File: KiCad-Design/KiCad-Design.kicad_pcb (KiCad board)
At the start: 2 copper layers, 35 x 35 mm, 66 parts, among them J1 USB_B_Micro, J2 Battery, J3 Ext, J4 OLED, Q1 SI2301, Q2 SI2301, Q3 SI2307CDS-T1-GE3, Q4 UMH3N, SW1 MCU BLE Adv, SW2 MCU FLASH, SW3 MCU RESET, U1 PMBT3904, U10 HDC1080, U2 BME280, U3 CP2104, U4 LTC4054ES5-4.2, U7 BME680, U8 AP2112K-3.3, U9 ttgo-32-micro-symbols

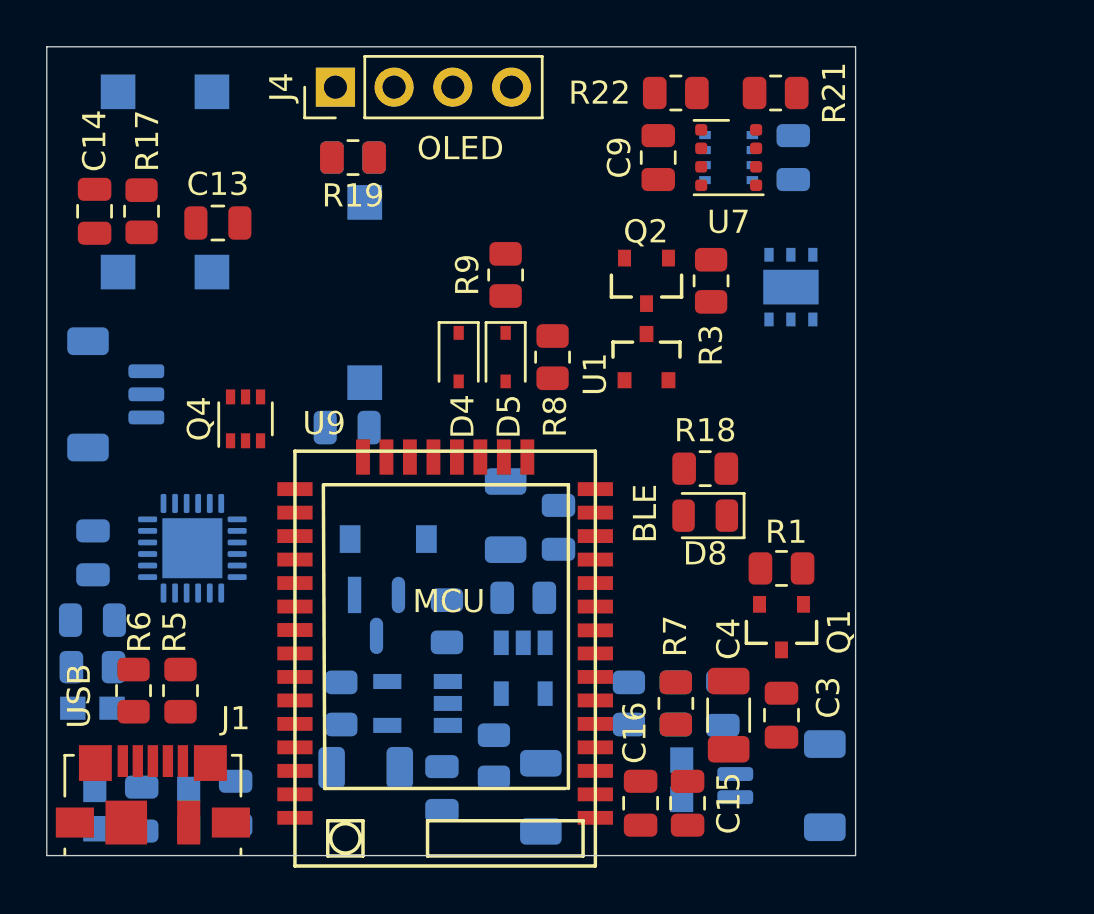
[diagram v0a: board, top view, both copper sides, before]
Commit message: PCB: Updating the PCB design file :)
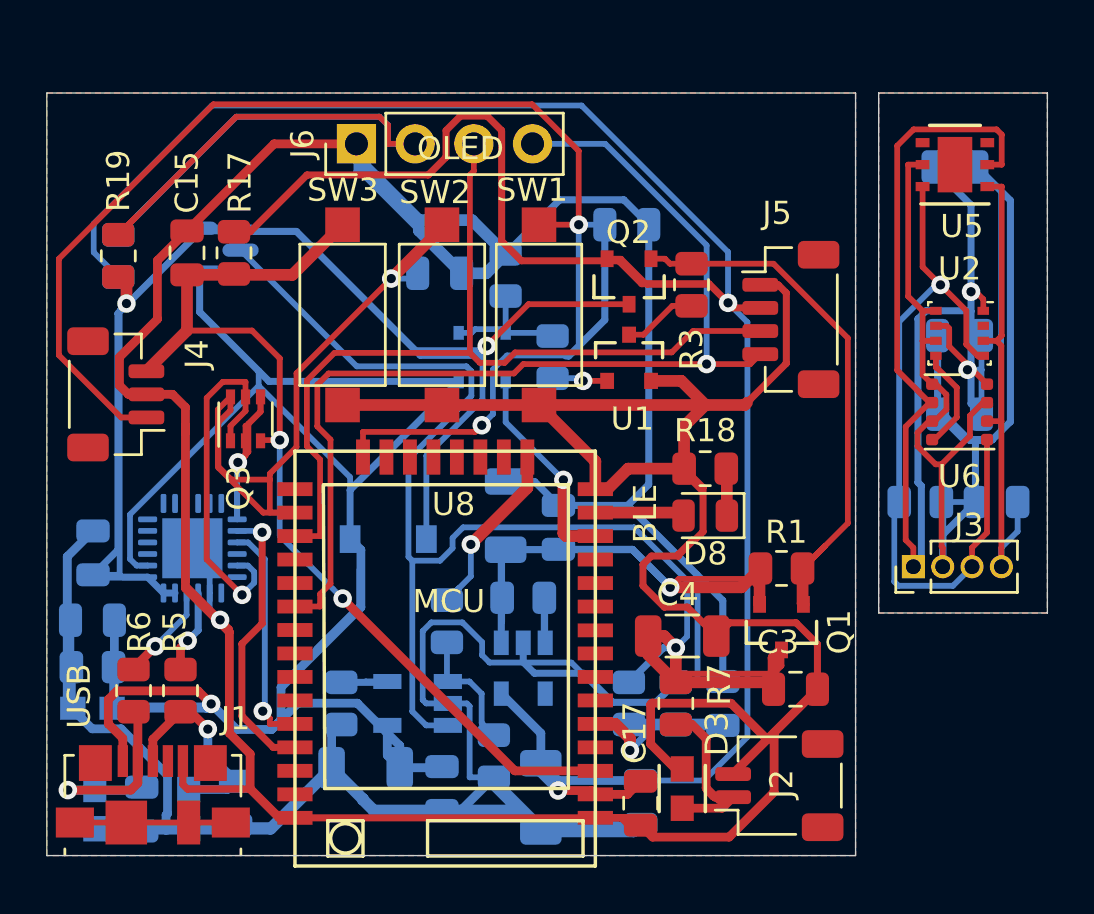
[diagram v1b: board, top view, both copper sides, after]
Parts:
- removed R21, R22: 4.7K, Resistor_SMD:R_0805_2012Metric
- removed U10: HDC1080, Package_SON:Texas_PWSON-N6
- removed the U7 at (254.5, 129.8)
- added C10: 100nF, Capacitor_SMD:C_0805_2012Metric, B.Cu at (264.5, 140.9)
- added J3: SENSOR, Connector_PinHeader_1.27mm:PinHeader_1x04_P1.27mm_Vertical, F.Cu at (262.5, 147.5)
- added J5: SENSORS, Connector_JST:JST_SH_BM04B-SRSS-TB_1x04-1MP_P1.00mm_Vertical, F.Cu at (257.2, 136.8)
- added R14: 4.7K, Resistor_SMD:R_0805_2012Metric, B.Cu at (266.1, 144.7)
- added R15: 4.7K, Resistor_SMD:R_0805_2012Metric, B.Cu at (262.8, 144.7)
- added U5: HDC1080, Package_SON:Texas_PWSON-N6, F.Cu at (264.3, 130.1)
- added U6: BME680, Package_LGA:Bosch_LGA-8_3x3mm_P0.8mm_ClockwisePinNumbering, F.Cu at (264.5, 140.8)
- C14: renamed from C13; moved to B.Cu
- C16: renamed from C15; moved to B.Cu
- C9, D4, D5, R8, R9: moved to B.Cu
- D3, J2, SW1, SW2, SW3, U2: moved to F.Cu
- J4: renamed from J3; moved to F.Cu
- moved Q4 17.2 mm to (232.5, 133.8), turned to 0 degrees
- moved C9 15.1 mm to (264.5, 137.5), turned to 0 degrees
- moved C13 15.0 mm to (250.1, 132.7), turned to 180 degrees
- moved U2 12.6 mm to (264.5, 137.4), turned to 270 degrees
- moved SW2 11.5 mm to (242.1, 136.6), turned to 270 degrees
- moved SW3 11.3 mm to (237.8, 136.6), turned to 270 degrees
- moved R19 11.0 mm to (228.1, 134.0), turned to 270 degrees
- moved R20 11.0 mm to (228.1, 134.0), turned to 270 degrees
- moved C14 9.84 mm to (242.0, 134.8), turned to 180 degrees
- moved SW1 7.60 mm to (246.3, 136.6), turned to 270 degrees
- moved C8 7.01 mm to (264.3, 130.2), turned to 180 degrees
- moved C15 4.39 mm to (231.1, 133.9)
- moved R17 4.39 mm to (233.1, 133.9)
- moved C4 3.97 mm to (252.5, 150.5), turned to 0 degrees
- moved J6 2.62 mm to (238.4, 129.2)
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- renumbered C10 to C11, C11 to C12, C12 to C13, C14 to C15, C16 to C17, C17 to C18, C18 to C19, C19 to C20, J4 to J6, Q4 to Q3, Q3 to Q4, U8 to U7, U9 to U8
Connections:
- C8 pad 1: GND -> SEN_VCC
- C8 pad 2: +3V3 -> SEN_GND
- C9 pad 1: GND -> SEN_VCC
- C9 pad 2: +3V3 -> SEN_GND
- U2 pad 1: GND -> SEN_GND
- U2 pad 2: +3V3 -> Net-(U2-Pad2)
- U2 pad 3: MCU_SDA -> SEN_SDA
- U2 pad 4: MCU_SCL -> SEN_SCL
- U2 pad 6: +3V3 -> SEN_VCC
- U2 pad 7: GND -> SEN_GND
- U2 pad 8: +3V3 -> SEN_VCC
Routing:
- net GND: track 0.00 -> 402.2 mm, vias 0 -> 1
- net +3V3: track 0.00 -> 113.6 mm, vias 0 -> 2
- net +5V: track 0.00 -> 102.4 mm, vias 0 -> 1
- net +VSW: track 0.00 -> 89.4 mm, vias 0 -> 2
- net SEN_VCC: track 0.00 -> 73.2 mm
- net +BATT: track 0.00 -> 71.2 mm, vias 0 -> 1
- net MCU_BLE_Adv: track 0.00 -> 66.0 mm, vias 0 -> 2
- net SEN_GND: track 0.00 -> 62.4 mm, vias 0 -> 2
- net MCU_RESET: track 0.00 -> 45.5 mm, vias 0 -> 2
- net MCU_SDA: track 0.00 -> 45.3 mm, vias 0 -> 1
- net MCU_SCL: track 0.00 -> 38.0 mm
- net VCC: track 0.00 -> 35.1 mm, vias 0 -> 1
- net Net-(J6-Pad2): track 0.00 -> 34.8 mm
- net SEN_SCL: track 0.00 -> 31.9 mm, vias 0 -> 1
- net MCU_FLASH: track 0.00 -> 31.0 mm, vias 0 -> 1
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- added copper zone on B.Cu, net GND
- added copper zone on F.Cu, net GND
- added copper zone on B.Cu, net SEN_GND
- added copper zone on F.Cu, net SEN_GND
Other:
- board size 35 x 35 mm -> 43.3 x 33 mm
- board text removed: "BATT"
- board text removed: "Ext"
